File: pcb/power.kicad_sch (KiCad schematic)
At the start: 77 parts, among them SW1 EVQPUJ02K, U1 AXP209, U100 MCIMX6Y7DVM09AB, U2 SY7208, U3 SY8120

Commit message: pcb: revise r0p1 design, ready for production
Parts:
- TH1: footprint Resistor_SMD:R_0603_1608Metric -> Resistor_SMD:R_0402_1005Metric
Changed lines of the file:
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@@
       (effects (font (size 1.27 1.27)) (justify left))
     )
-    (property "Footprint" "Resistor_SMD:R_0603_1608Metric" (id 2) (at 63.5 88.9 0)
+    (property "Footprint" "Resistor_SMD:R_0402_1005Metric" (id 2) (at 63.5 88.9 0)
       (effects (font (size 1.27 1.27)) hide)
     )

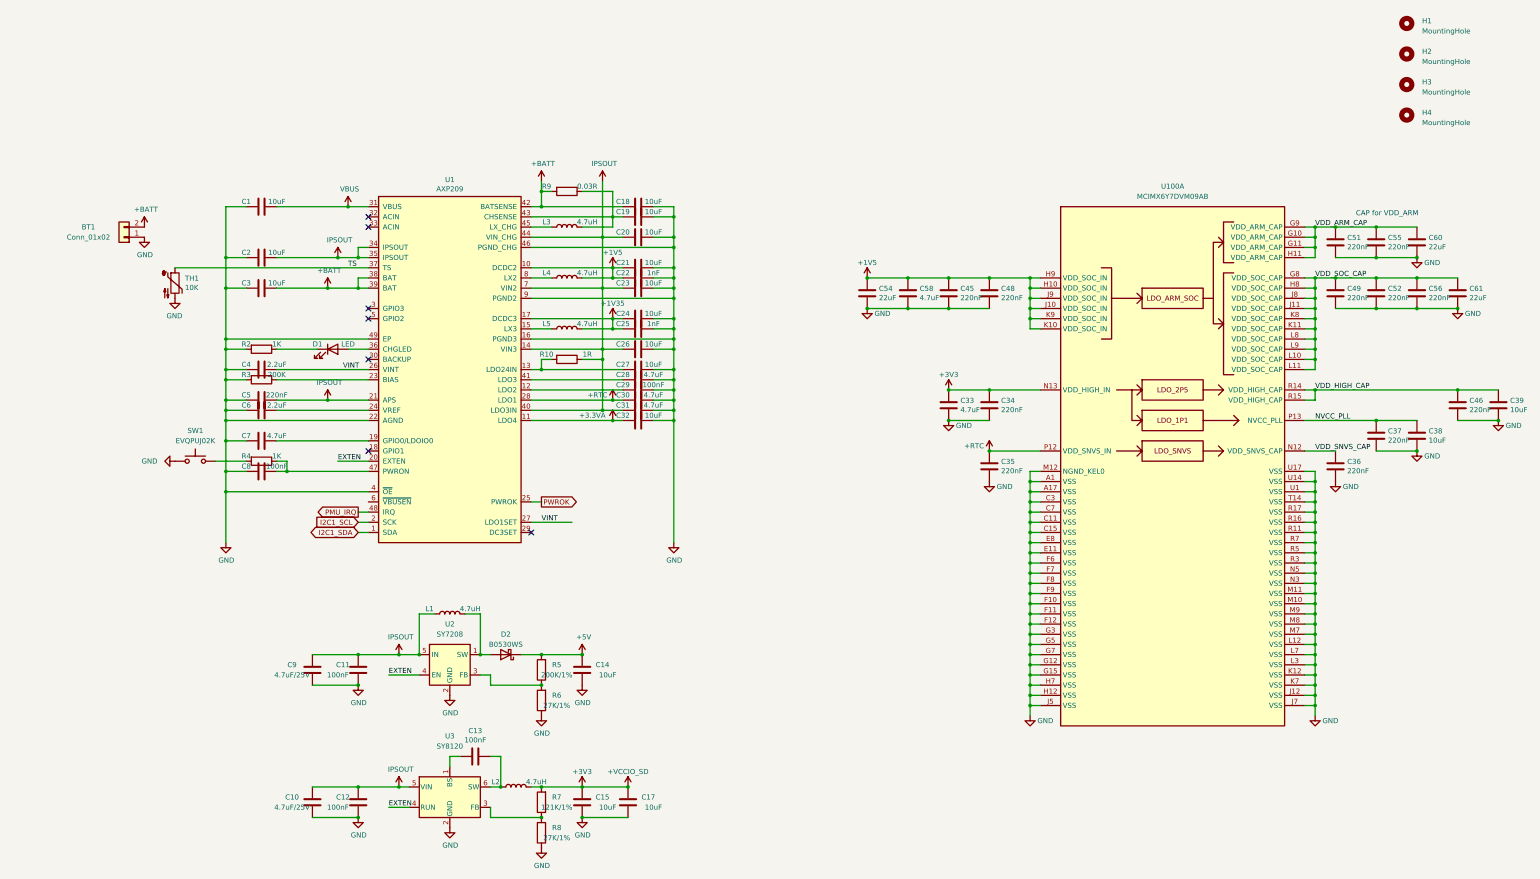
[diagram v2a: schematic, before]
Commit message: pcb: getting ready for r0.2 production
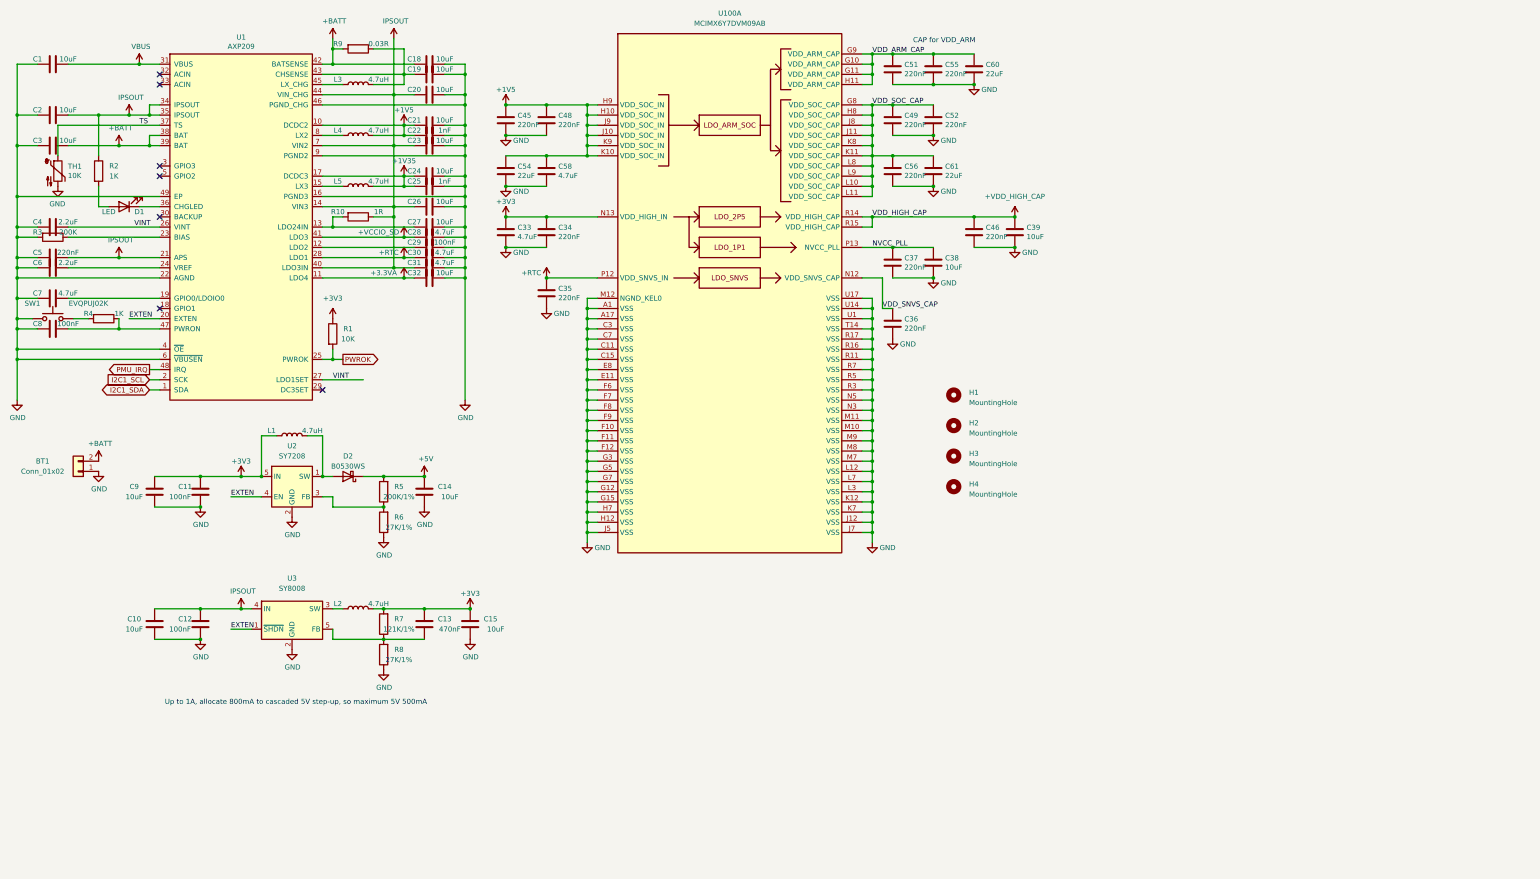
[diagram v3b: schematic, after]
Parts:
- removed C17: 10uF, Capacitor_SMD:C_0603_1608Metric, symbol Device:C
- removed U3: SY8120, Package_TO_SOT_SMD:TSOT-23-6, symbol symbols:SY8120
- added R1: 10K, Resistor_SMD:R_0402_1005Metric, symbol Device:R
- added U3: SY8008, Package_TO_SOT_SMD:TSOT-23-5, symbol symbols:SY8008
- C10, C9: value 4.7uF/25V -> 10uF
- C13: value 100nF -> 470nF
- TH1: footprint Resistor_SMD:R_0402_1005Metric -> Resistor_SMD:R_0603_1608Metric
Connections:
- net +3V3: now also C11.2, C13.2, C9.2, L1.1, U2.5 (IN), R1.1
- net EXTEN: now also U3.1 (~{SHDN})
- net GND: now also U1.6 (~{VBUSEN}), U3.2 (GND); no longer R2.2
- net IPSOUT: now also R2.1, U3.4 (IN); no longer C11.2, C9.2, L1.1, U2.5 (IN)
- net PWROK: now also R1.2
- net at R7.1, R8.2: now also C13.1, U3.5 (FB)
- net at L2.1: now also U3.3 (SW); no longer C13.1
- net +VCCIO_SD: now reaches C28.2, U1.41 (LDO3)
- net at D1.1 (K): now also U1.36 (CHGLED); no longer R2.1
- net at D1.2 (A): now also R2.2; no longer U1.36 (CHGLED)
- net VDD_HIGH_CAP renamed +VDD_HIGH_CAP
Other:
- note added: "Up to 1A, allocate 800mA to cascaded 5V step-up, so maximum 5V 500mA"
- moved on the sheet: BT1, C1, C10, C11, C12, C14, C15, C18, C19, C2, C20, C21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
